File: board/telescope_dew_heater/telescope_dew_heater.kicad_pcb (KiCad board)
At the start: 2 copper layers, 58 x 100 mm, 39 parts, among them J1 RCA1, J2 RCA1, J3 RCA1, J4 RCA1, J5 Barrel_Jack, Q1 Q_NMOS_GDS, Q2 Q_NMOS_GDS, Q3 Q_NMOS_GDS, Q4 Q_NMOS_GDS, SW1 SW_DPDT_x2, U1 NE555P, U2 NE555P, U3 NE555P, U4 NE555P

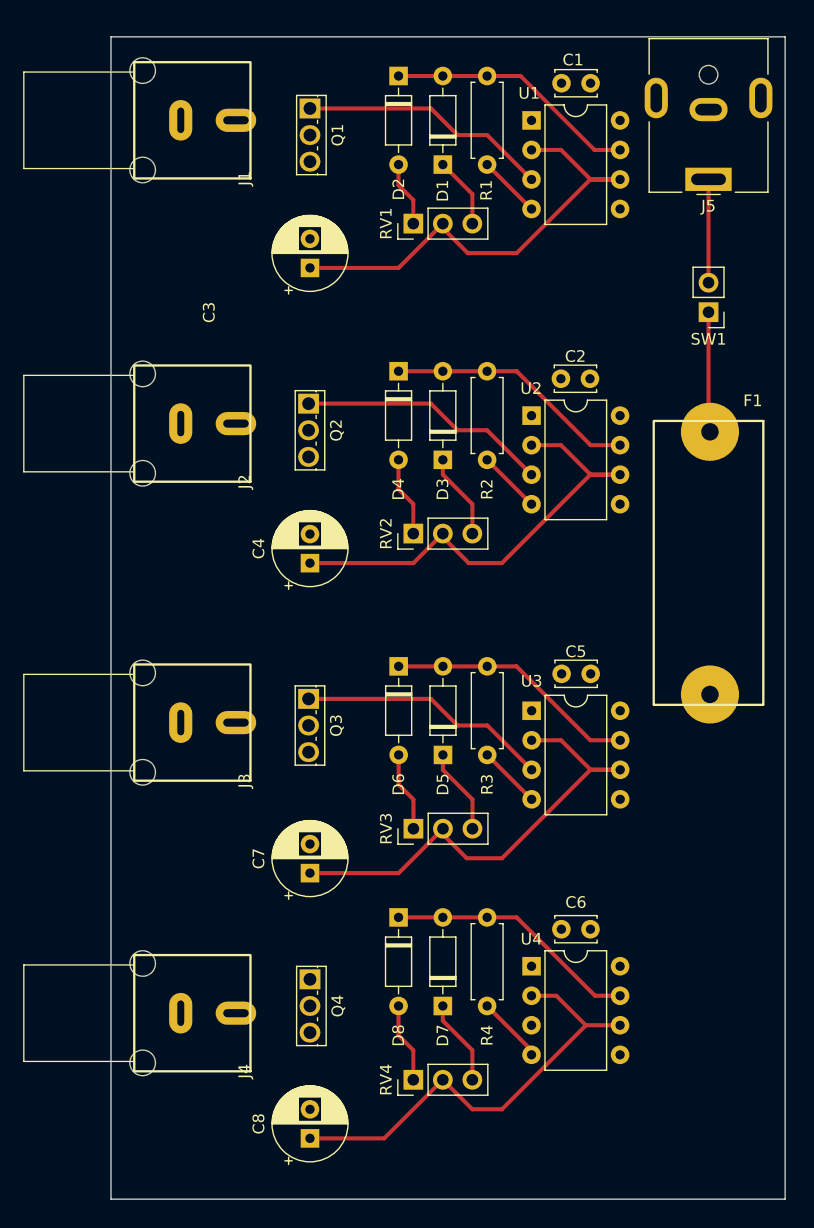
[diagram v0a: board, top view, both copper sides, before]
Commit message: Production Commit
AS SUBMITTED TO PCBWAY
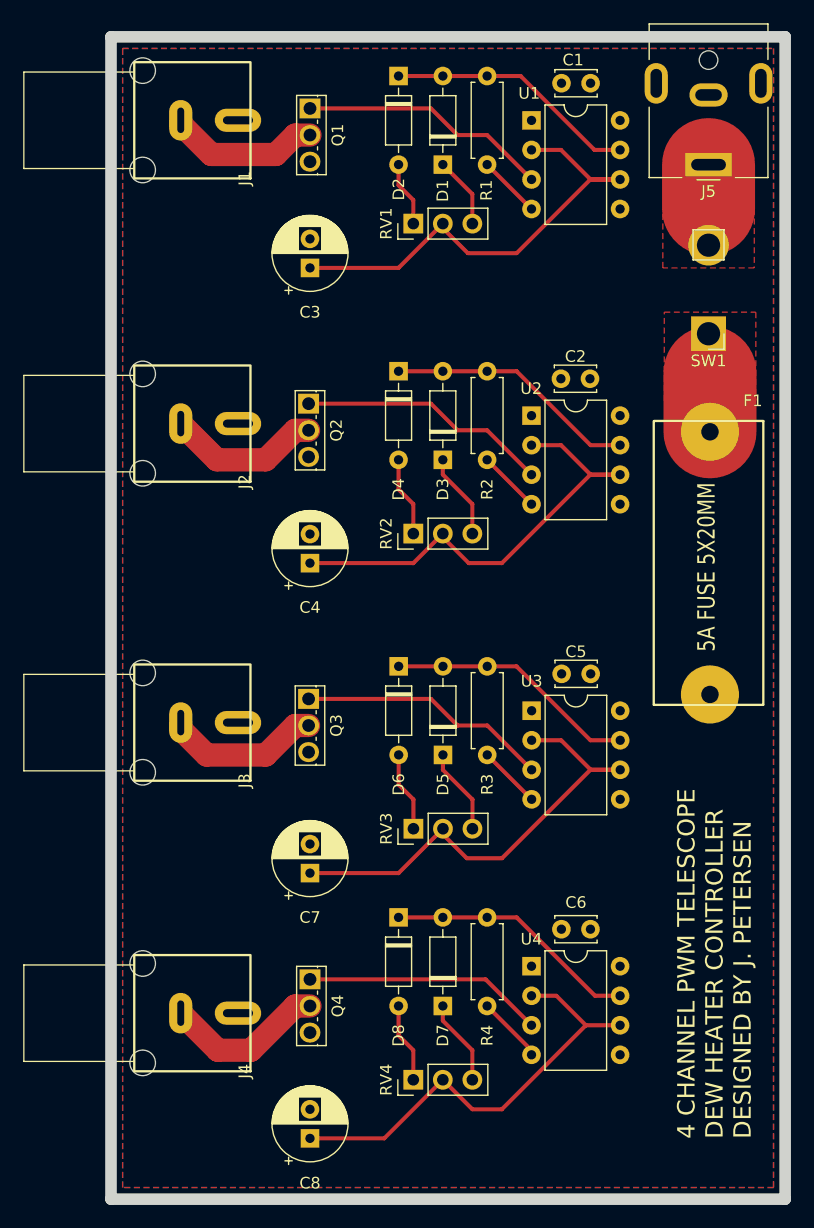
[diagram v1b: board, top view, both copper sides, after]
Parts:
- moved SW1 1.86 mm to (105.4, 61.5)
- moved J5 1.26 mm to (105.4, 47.0)
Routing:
- net Net-(Q4-G): track 0.00 -> 20.7 mm
- net Net-(J4-Ext): track 0.00 -> 14.0 mm
- net Net-(J3-Ext): track 0.00 -> 13.5 mm
- net Net-(J2-Ext): track 0.00 -> 13.3 mm
- net Net-(J1-Ext): track 0.00 -> 13.2 mm
- net Net-(SW1A-A): track 10.3 -> 5.26 mm
- net Net-(SW1A-B): track 8.89 -> 3.82 mm
- net +12V: track 22.0 -> 22.6 mm
- added copper zone on F.Cu, net +12V
- added copper zone on B.Cu, net GND
- added copper zone on F.Cu, net Net-(SW1A-A)
- added copper zone on F.Cu, net Net-(SW1A-B)
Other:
- board text added: "4 CHANNEL PWM TELESCOPE DEW HEATER CONTROLLER DESIGNED BY J. PETERSEN"
- board text added: "5A FUSE 5X20MM"
